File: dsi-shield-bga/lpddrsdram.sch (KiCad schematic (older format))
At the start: 1 part, among them U2 K4X1G163PE

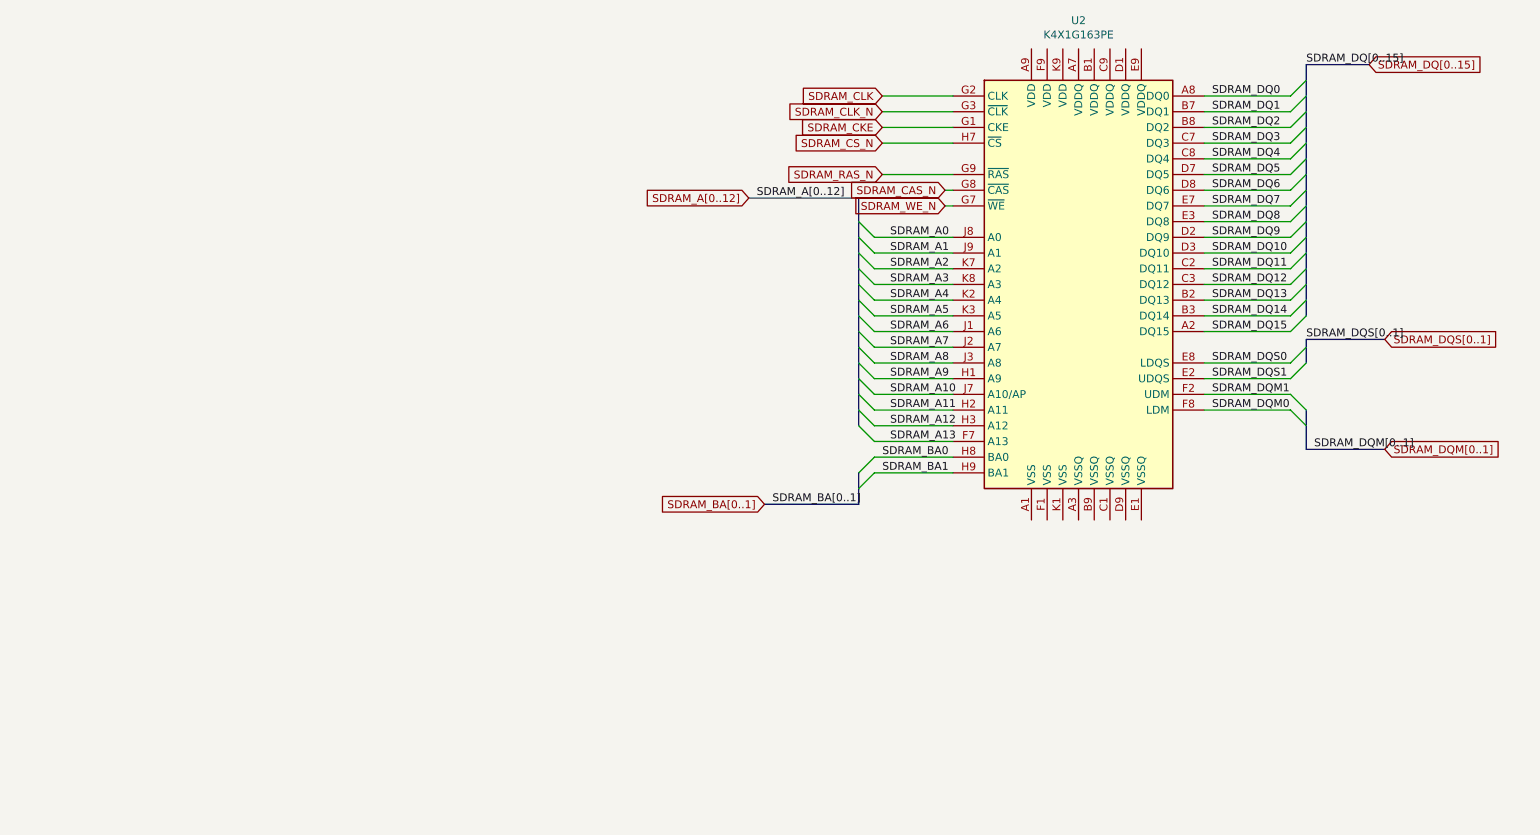
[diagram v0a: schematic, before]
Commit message: 20200808
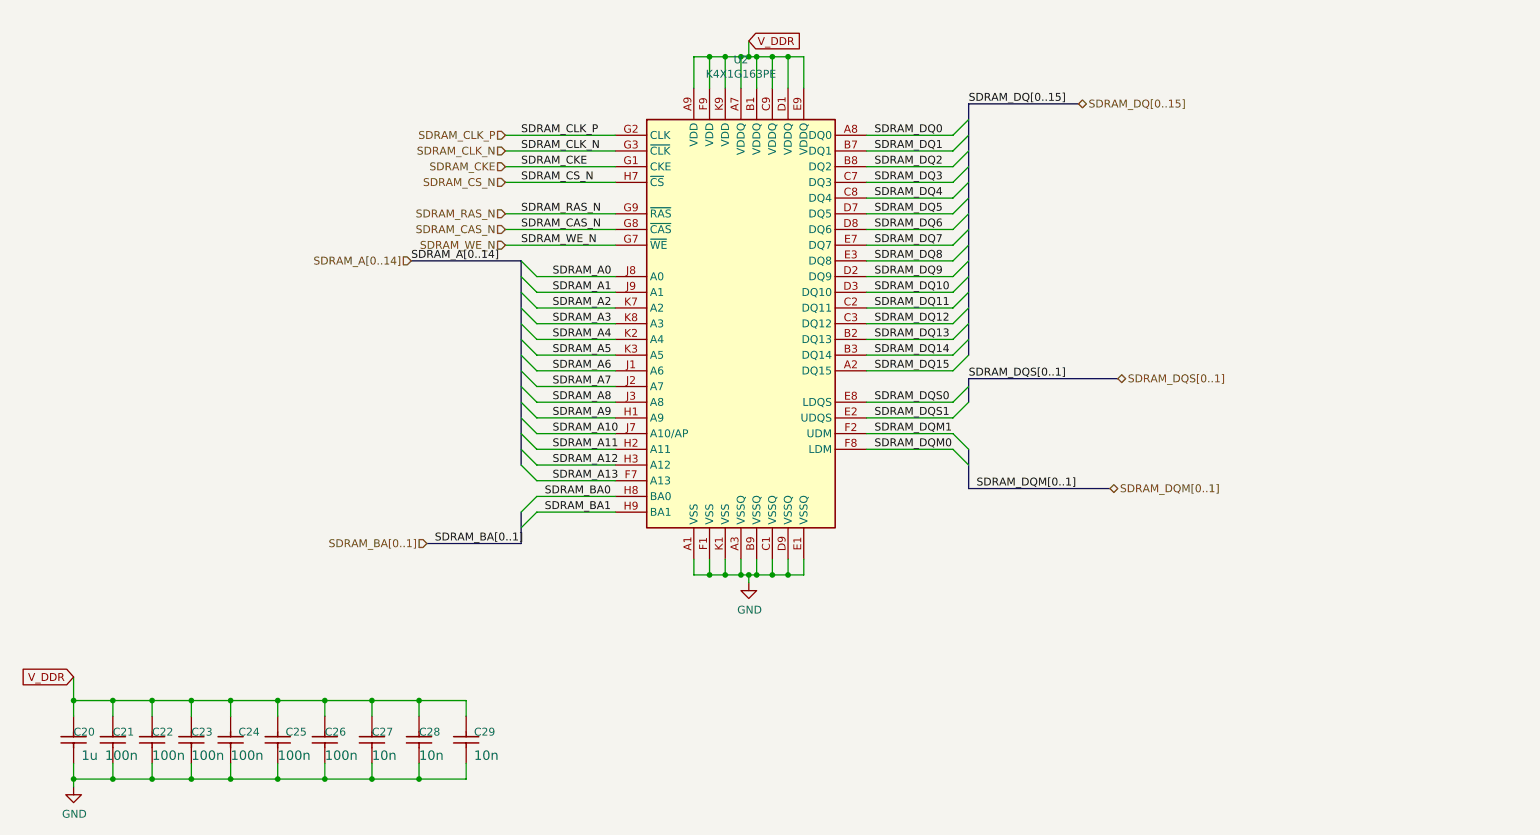
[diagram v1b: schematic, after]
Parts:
- added C20: 1u, Capacitor_SMD:C_0402_1005Metric, symbol dsi_shield:Cap
- added C21, C22, C23, C24, C25, C26: 100n, Capacitor_SMD:C_0402_1005Metric, symbol dsi_shield:Cap
- added C27, C28, C29: 10n, Capacitor_SMD:C_0402_1005Metric, symbol dsi_shield:Cap
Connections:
- net GND: now reaches U2.A1 (VSS)
- net GND: now also U2.A3 (VSSQ), U2.B9 (VSSQ), U2.C1 (VSSQ), U2.D9 (VSSQ), U2.E1 (VSSQ), U2.F1 (VSS), U2.K1 (VSS), C20.2, C21.2, C22.2, C23.2, C24.2, C25.2, C26.2, C27.2, C28.2, C29.2
- net V_DDR: now reaches U2.A7 (VDDQ)
- net V_DDR: now also U2.A9 (VDD), U2.B1 (VDDQ), U2.C9 (VDDQ), U2.D1 (VDDQ), U2.E9 (VDDQ), U2.F9 (VDD), U2.K9 (VDD), C20.1, C21.1, C22.1, C23.1, C24.1, C25.1, C26.1, C27.1, C28.1, C29.1
- net SDRAM_CLK renamed SDRAM_CLK_P
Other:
- moved on the sheet: U2
